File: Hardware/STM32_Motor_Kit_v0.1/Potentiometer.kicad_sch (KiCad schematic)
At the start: 8 parts

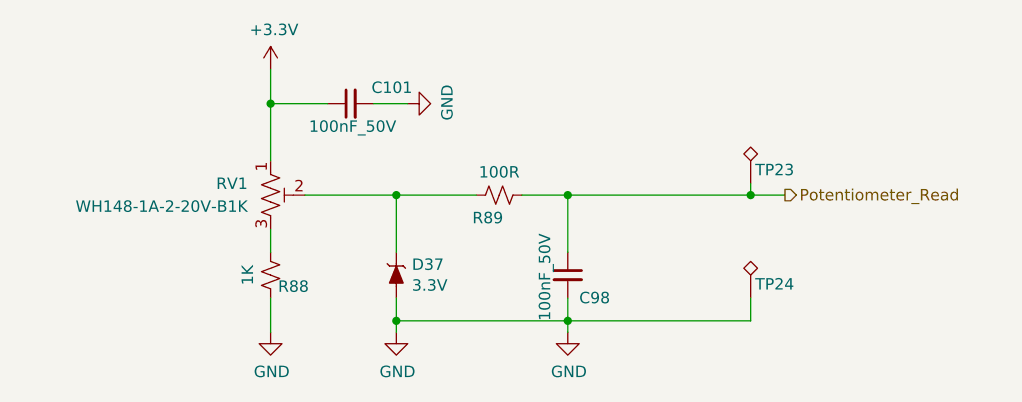
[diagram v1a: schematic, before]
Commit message: 12.01.2025
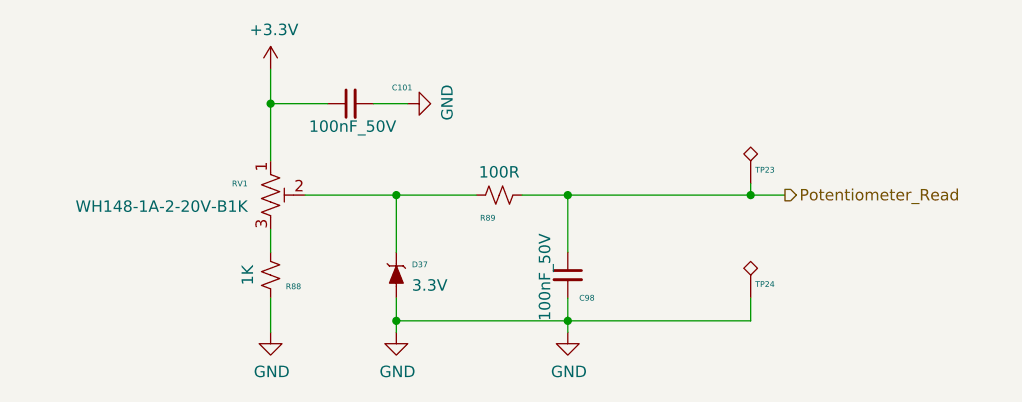
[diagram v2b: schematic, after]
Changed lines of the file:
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@@
 			(effects
 				(font
-					(size 1.27 1.27)
+					(face "Arial")
+					(size 0.635 0.635)
 				)
 				(hide yes)
@@
 			(effects
 				(font
-					(size 1.27 1.27)
+					(face "Arial")
+					(size 0.635 0.635)
 				)
 				(justify left)
@@
 			(effects
 				(font
-					(size 1.27 1.27)
+					(face "Arial")
+					(size 0.635 0.635)
 				)
 				(hide yes)
@@
 			(effects
 				(font
-					(size 1.27 1.27)
+					(face "Arial")
+					(size 0.635 0.635)
 				)
 				(justify right)
@@
 			(effects
 				(font
-					(size 1.27 1.27)
+					(face "Arial")
+					(size 0.635 0.635)
 				)
 			)
@@
 			(effects
 				(font
-					(size 1.27 1.27)
+					(face "Arial")
+					(size 0.635 0.635)
 				)
 				(justify left)
@@
 			(effects
 				(font
-					(size 1.27 1.27)
+					(face "Arial")
+					(size 0.635 0.635)
 				)
 				(hide yes)
@@
 			(effects
 				(font
-					(size 1.27 1.27)
+					(face "Arial")
+					(size 0.635 0.635)
 				)
 			)
@@
 			(effects
 				(font
-					(size 1.27 1.27)
+					(face "Arial")
+					(size 0.635 0.635)
 				)
 				(hide yes)
@@
 			(effects
 				(font
-					(size 1.27 1.27)
+					(face "Arial")
+					(size 0.635 0.635)
 				)
 				(justify left)
@@
 			(effects
 				(font
-					(size 1.27 1.27)
+					(face "Arial")
+					(size 0.635 0.635)
 				)
 				(justify left)
@@
 			(effects
 				(font
-					(size 1.27 1.27)
+					(face "Arial")
+					(size 0.635 0.635)
 				)
 				(hide yes)
@@
 			(effects
 				(font
-					(size 1.27 1.27)
+					(face "Arial")
+					(size 0.635 0.635)
 				)
 				(justify left)
